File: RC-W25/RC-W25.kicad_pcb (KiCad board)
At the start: 2 copper layers, 40.3 x 100 mm, 55 parts, among them J1 USB_C_Receptacle_USB2.0_14P, P1 JST CONN, P2 JST CONN, Q1 NMOS, SW1 Button, SW2 Button, SW3 YTSPS-22E58LM, SW4 Button, U1 ESP32-C6-WROOM-1, U2 MCP73831-5-OT, U3 AP62300TWU, U4 TMAG5253

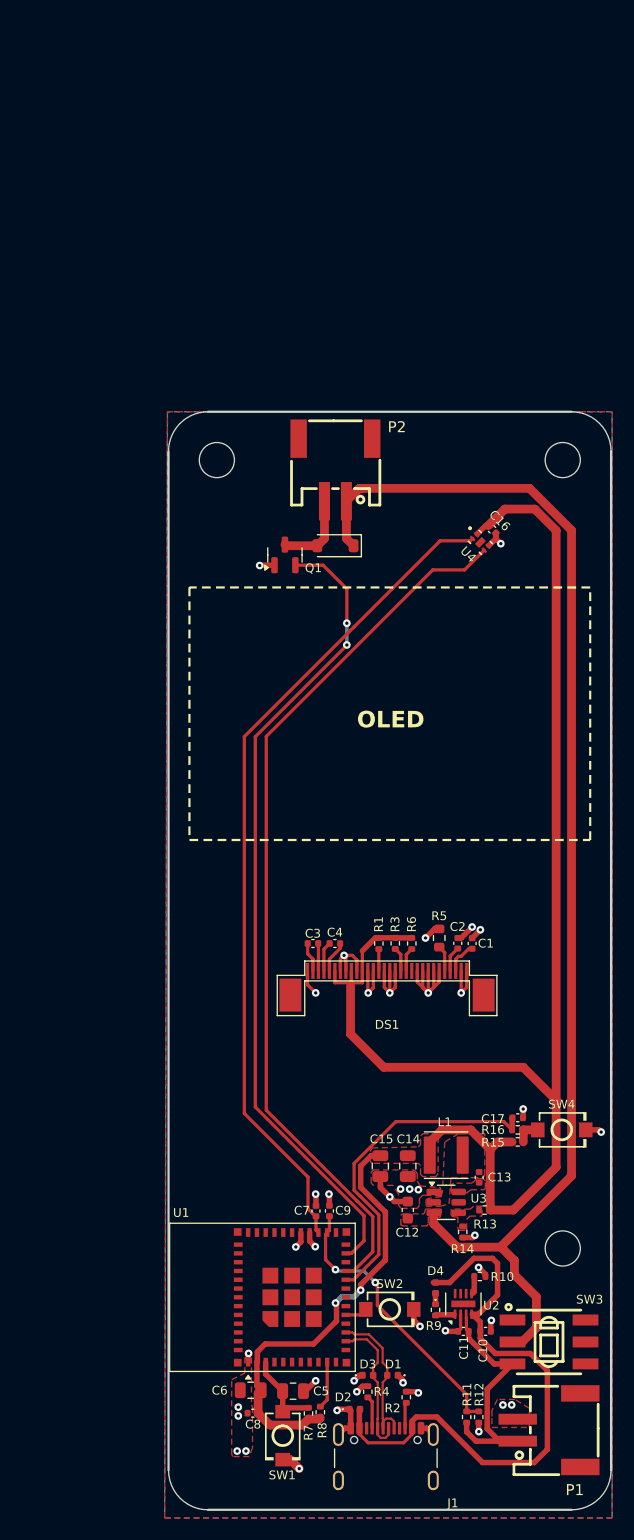
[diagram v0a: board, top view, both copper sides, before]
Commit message: crc v1
board complete and ready for assembly setup!
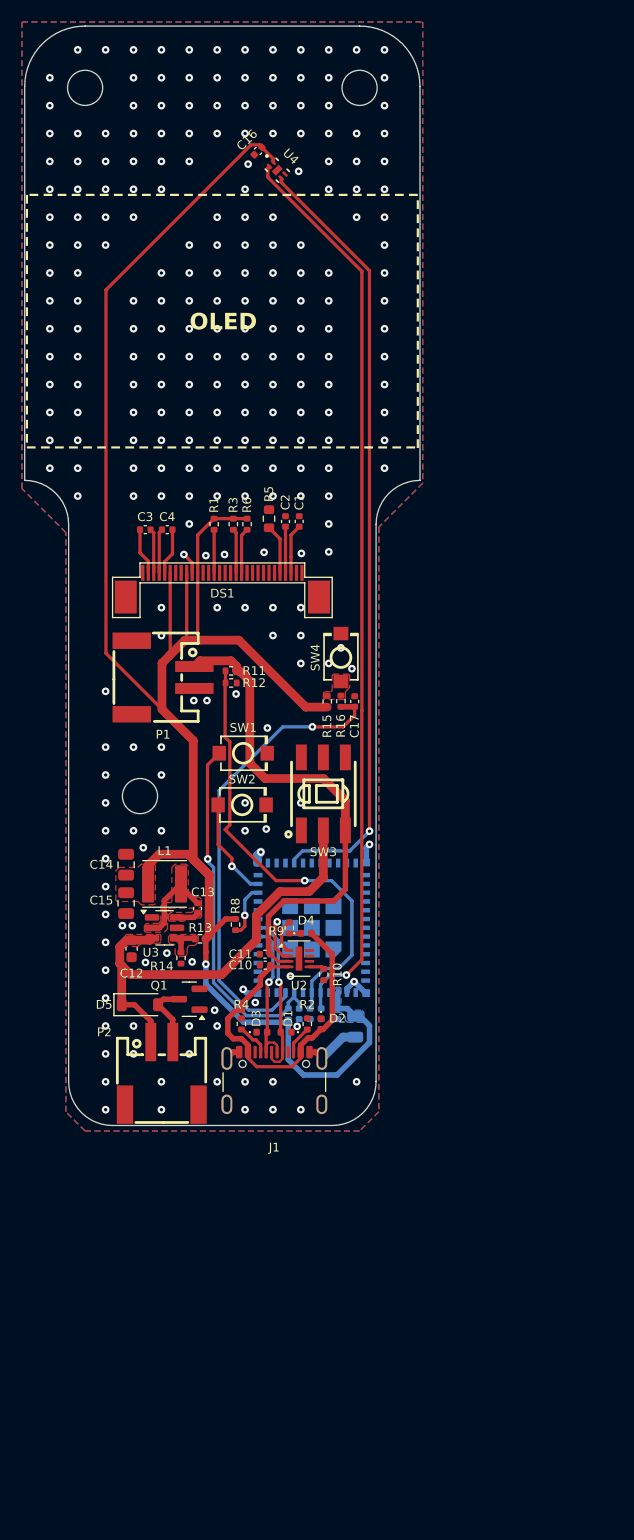
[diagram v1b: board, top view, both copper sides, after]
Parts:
- C5: value 1uF -> 100nF; footprint Capacitor_SMD:C_0805_2012Metric -> Capacitor_SMD:C_0402_1005Metric; moved to B.Cu
- C6: value 22uF -> 100nF; footprint Capacitor_SMD:C_0805_2012Metric -> Capacitor_SMD:C_0402_1005Metric; moved to B.Cu
- C7, C9, R7: moved to B.Cu
- C8: value 100nF -> 22uF; footprint Capacitor_SMD:C_0402_1005Metric -> Capacitor_SMD:C_0805_2012Metric; moved to B.Cu
- U1: value ESP32-C6-WROOM-1 -> ESP32-C6-MINI-1; moved to B.Cu
- moved H1 107.3 mm to (137.5, 30.5)
- moved P1 77.0 mm to (119.6, 84.2), turned to -90 degrees
- moved R11 71.3 mm to (125.8, 83.6), turned to 180 degrees
- moved R12 70.6 mm to (125.8, 84.7), turned to 0 degrees
- moved SW1 62.3 mm to (126.9, 91.1), turned to 0 degrees
- moved P2 57.2 mm to (119.5, 120.2), turned to 0 degrees
- moved H2 55.1 mm to (112.5, 30.5)
- moved SW3 54.0 mm to (134.2, 94.8), turned to 90 degrees
- moved SW2 47.9 mm to (126.8, 95.8)
- moved SW4 47.5 mm to (135.8, 82.4), turned to 90 degrees
- moved D5 45.4 mm to (117.5, 114.0), turned to 0 degrees
- moved R8 45.1 mm to (126.2, 106.7), turned to -90 degrees
- moved R15 43.7 mm to (134.6, 86.4), turned to 90 degrees
- moved R16 42.2 mm to (135.8, 86.4), turned to -90 degrees
- moved C1 41.5 mm to (132.0, 70.0)
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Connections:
- C5 pad 1: /RC_Connections/RESET -> ADC_HALLEFFECT1
- C6 pad 1: +3.3V -> /RC_Connections/RESET
- C7 pad 1: ADC_HALLEFFECT1 -> ADC_BATTERYPERCENT
- C9 pad 1: ADC_BATTERYPERCENT -> +3.3V
- R8 pad 2: Net-(U1-GPIO8) -> Net-(U1-IO8)
- U1 pad 10: Net-(U1-GPIO8) -> unconnected-(U1-IO5-Pad10)
- U1 pad 11: unconnected-(U1-GPIO10-Pad11) -> GND
- U1 pad 12: unconnected-(U1-GPIO11-Pad12) -> GND
- U1 pad 13: USB_D- -> GND
- U1 pad 14: USB_D+ -> GND
- U1 pad 16: /RC_Connections/FLASH -> unconnected-(U1-IO7-Pad16)
- U1 pad 17: unconnected-(U1-GPIO19-Pad17) -> USB_D-
- U1 pad 18: unconnected-(U1-GPIO20-Pad18) -> USB_D+
- U1 pad 2: +3.3V -> GND
- U1 pad 20: GPIO_MODE -> unconnected-(U1-IO15-Pad20)
- U1 pad 21: GPIO_EN1 -> unconnected-(U1-NC-Pad21)
- U1 pad 22: unconnected-(U1-NC-Pad22) -> Net-(U1-IO8)
- U1 pad 23: GPIO_RUMBLE_CNTL -> /RC_Connections/FLASH
- U1 pad 26: ADC_BATTERYPERCENT -> unconnected-(U1-IO20-Pad26)
- U1 pad 27: ADC_HALLEFFECT1 -> unconnected-(U1-IO21-Pad27)
- U1 pad 28: GND -> GPIO_EN1
- U1 pad 29: GND -> unconnected-(U1-IO23-Pad29)
- U1 pad 3: /RC_Connections/RESET -> +3.3V
- U1 pad 30: (no net) -> unconnected-(U1-RXD0-Pad30)
- U1 pad 31: (no net) -> unconnected-(U1-TXD0-Pad31)
- U1 pad 32: (no net) -> unconnected-(U1-NC-Pad32)
- U1 pad 33: (no net) -> unconnected-(U1-NC-Pad33)
- U1 pad 34: (no net) -> unconnected-(U1-NC-Pad34)
- U1 pad 35: (no net) -> unconnected-(U1-NC-Pad35)
- U1 pad 36: (no net) -> GND
- U1 pad 37: (no net) -> GND
- U1 pad 38: (no net) -> GND
- U1 pad 39: (no net) -> GND
- U1 pad 40: (no net) -> GND
- U1 pad 41: (no net) -> GND
- U1 pad 42: (no net) -> GND
- U1 pad 43: (no net) -> GND
- U1 pad 44: (no net) -> GND
- U1 pad 45: (no net) -> GND
- U1 pad 46: (no net) -> GND
- U1 pad 47: (no net) -> GND
- U1 pad 48: (no net) -> GND
- U1 pad 49: (no net) -> GND
- U1 pad 5: unconnected-(U1-MTDI/GPIO5/ADC1_CH5-Pad5) -> ADC_HALLEFFECT1
- U1 pad 50: (no net) -> GND
- U1 pad 51: (no net) -> GND
- U1 pad 52: (no net) -> GND
- U1 pad 53: (no net) -> GND
- U1 pad 6: unconnected-(U1-MTCK/GPIO6/ADC1_CH6-Pad6) -> ADC_BATTERYPERCENT
- U1 pad 8: unconnected-(U1-GPIO0/ADC1_CH0/XTAL_32K_P-Pad8) -> /RC_Connections/RESET
- U1 pad 9: unconnected-(U1-GPIO1/ADC1_CH1/XTAL_32K_N-Pad9) -> GPIO_MODE
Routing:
- net GPIO_RUMBLE_CNTL: track 74.6 -> 0.00 mm, vias 2 -> 0
- net +VBAT: track 114.0 -> 42.0 mm
- net GND: track 76.2 -> 19.9 mm, vias 41 -> 256
- net /RC_Connections/RESET: track 7.65 -> 33.2 mm, vias 0 -> 1
- net Net-(P1-Pin_1): track 21.5 -> 45.4 mm
- net +USB5V: track 53.5 -> 32.4 mm
- net ADC_BATTERYPERCENT: track 26.0 -> 41.2 mm, vias 2 -> 1
- net GPIO_MODE: track 30.6 -> 42.6 mm, vias 0 -> 1
- net +3.3V: track 168.8 -> 180.3 mm, vias 2 -> 1
- net GPIO_EN1: track 81.0 -> 71.1 mm, vias 0 -> 1
- net Net-(U3-SW): track 0.00 -> 7.85 mm
- net /RC_Connections/FLASH: track 2.02 -> 9.16 mm, vias 0 -> 1
- net ADC_HALLEFFECT1: track 76.3 -> 82.8 mm, vias 0 -> 1
- net Net-(U1-IO8): track 0.00 -> 5.04 mm, vias 0 -> 1
- net Net-(U1-GPIO8): track 4.31 -> 0.00 mm
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- added copper zone on B.Cu, net +3.3V
- added copper zone on F.Cu, net Net-(R15-Pad2)
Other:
- board size 40.3 x 100 mm -> 36 x 100.1 mm
